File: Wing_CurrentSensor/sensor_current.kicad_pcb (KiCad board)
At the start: 2 copper layers, 50.8 x 22.9 mm, 25 parts, among them J1 feather long, J2 feather short, J3 SJ-3524-SMT, J4 Analog Selection, U1 TL084, U2 AD8226

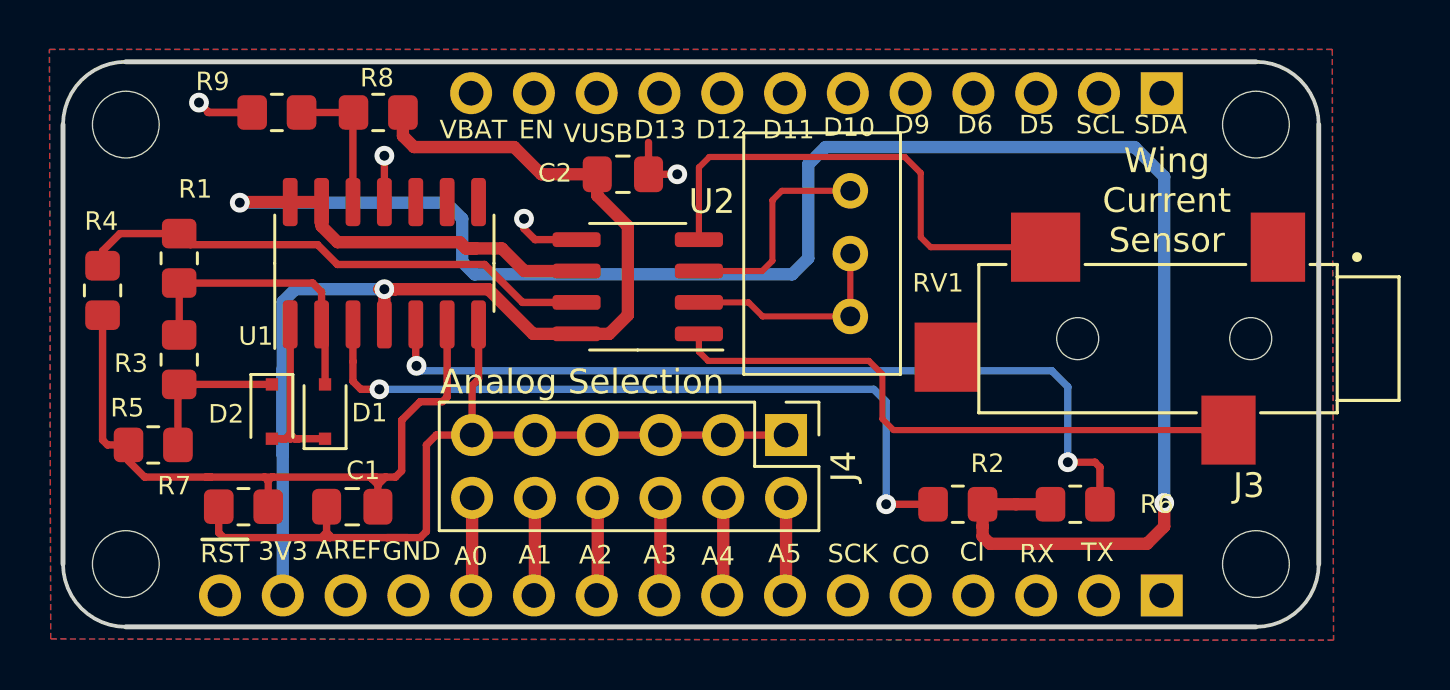
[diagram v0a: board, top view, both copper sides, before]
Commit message: Add_Connector
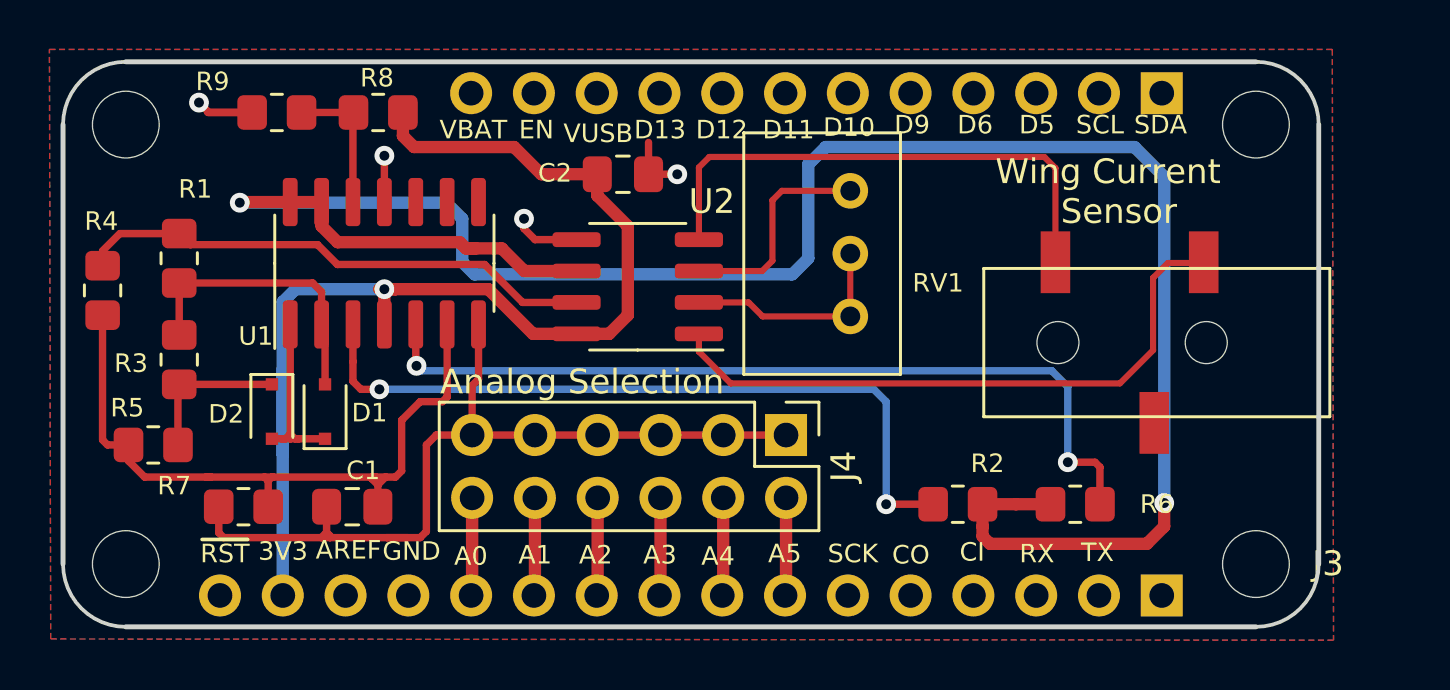
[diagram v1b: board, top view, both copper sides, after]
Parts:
- moved J3 4.50 mm to (159.2, 104.8)
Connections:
- J3 pad 1: Net-(J3-Pad1) -> GND
- J3 pad 2: /IN+ -> Net-(J3-Pad2)
- J3 pad 3: /IN- -> /IN+
- U2 pad 1: /IN- -> GND
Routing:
- net GND: track 11.2 -> 36.6 mm
- net /IN-: track 24.5 -> 0.00 mm
- net /IN+: track 20.2 -> 21.5 mm
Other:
- net class Default: trace_width 0.3 -> 0.25
